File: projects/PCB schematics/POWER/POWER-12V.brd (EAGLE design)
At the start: 160 x 100 mm, 0 parts

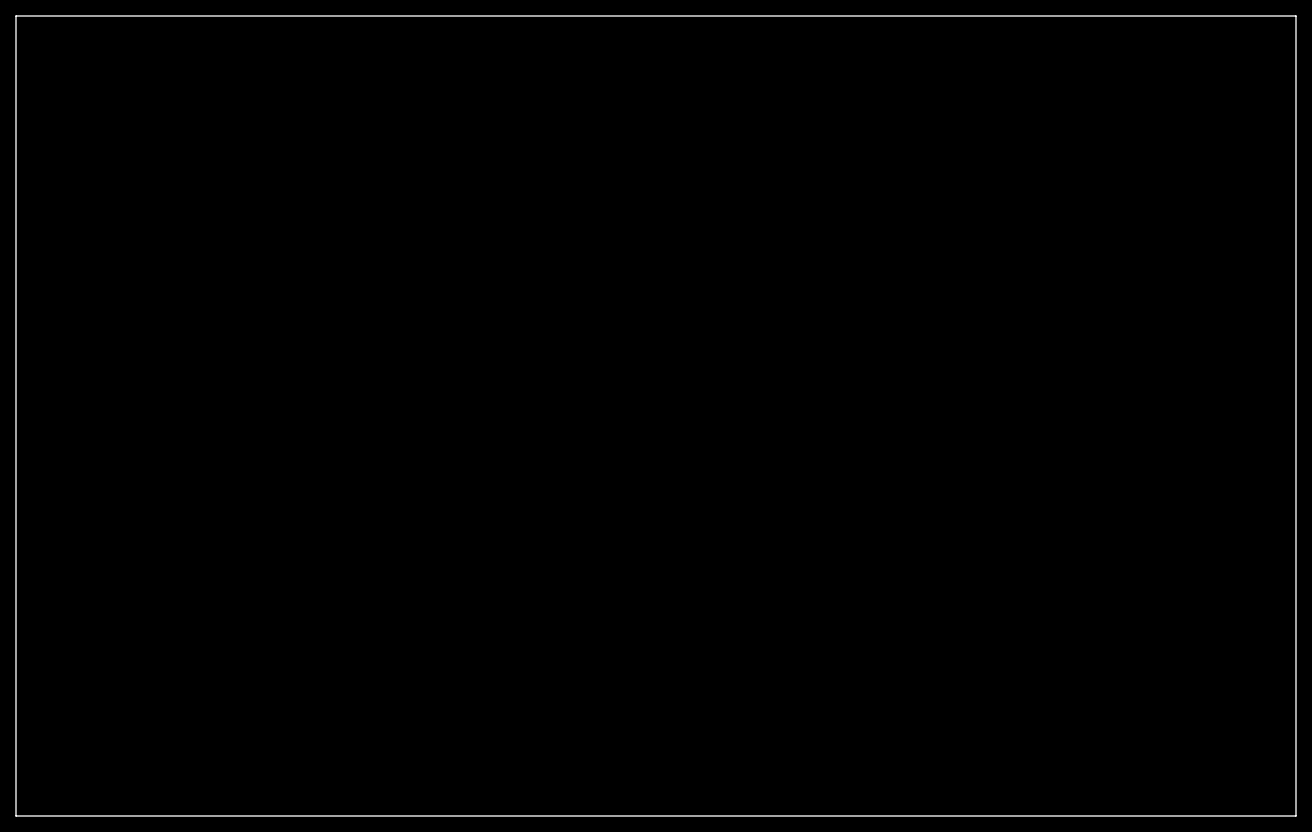
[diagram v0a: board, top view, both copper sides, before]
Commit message: RTDS - Rev A.
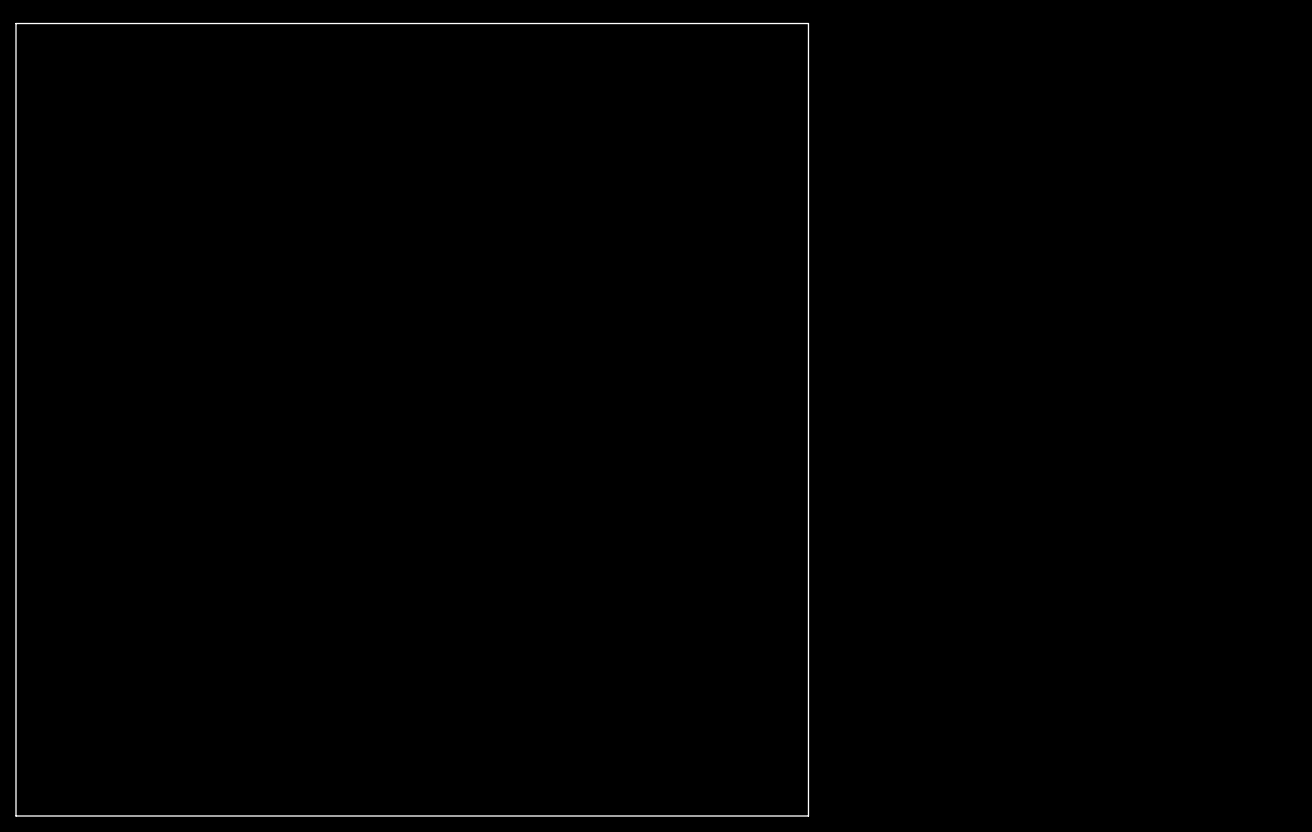
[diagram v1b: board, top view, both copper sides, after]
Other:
- board size 160 x 100 mm -> 99.1 x 99.1 mm
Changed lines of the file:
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@@
 <?xml version="1.0" encoding="utf-8"?>
 <!DOCTYPE eagle SYSTEM "eagle.dtd">
-<eagle version="9.3.2">
+<eagle version="9.4.0">
 <drawing>
 <settings>
@@
 <setting verticaltext="up"/>
 </settings>
-<grid distance="50" unitdist="mil" unit="mil" style="lines" multiple="1" display="no" altdistance="5" altunitdist="mil" altunit="mil"/>
+<grid distance="50" unitdist="mil" unit="mil" style="lines" multiple="1" display="yes" altdistance="1" altunitdist="mil" altunit="mil"/>
 <layers>
 <layer number="1" name="Top" color="4" fill="1" visible="yes" active="yes"/>
@@
 <board>
 <plain>
-<wire x1="0" y1="0" x2="160" y2="0" width="0" layer="20"/>
-<wire x1="160" y1="0" x2="160" y2="100" width="0" layer="20"/>
-<wire x1="160" y1="100" x2="0" y2="100" width="0" layer="20"/>
-<wire x1="0" y1="100" x2="0" y2="0" width="0" layer="20"/>
+<wire x1="0" y1="0" x2="99.06" y2="0" width="0" layer="20"/>
+<wire x1="99.06" y1="0" x2="99.06" y2="99.06" width="0" layer="20"/>
+<wire x1="99.06" y1="99.06" x2="0" y2="99.06" width="0" layer="20"/>
+<wire x1="0" y1="99.06" x2="0" y2="0" width="0" layer="20"/>
 </plain>
 <attributes>
@@
 </class>
 </classes>
-<designrules name="default">
-<description language="de">&lt;b&gt;EAGLE Design Rules&lt;/b&gt;
-&lt;p&gt;
-Die Standard-Design-Rules sind so gewählt, dass sie für
-die meisten Anwendungen passen. Sollte ihre Platine
-besondere Anforderungen haben, treffen Sie die erforderlichen
-Einstellungen hier und speichern die Design Rules unter
-einem neuen Namen ab.</description>
+<designrules name="default *">
 <description language="en">&lt;b&gt;EAGLE Design Rules&lt;/b&gt;
 &lt;p&gt;
@@
 <param name="mtCopper" value="0.035mm 0.035mm 0.035mm 0.035mm 0.035mm 0.035mm 0.035mm 0.035mm 0.035mm 0.035mm 0.035mm 0.035mm 0.035mm 0.035mm 0.035mm 0.035mm"/>
 <param name="mtIsolate" value="1.5mm 0.15mm 0.2mm 0.15mm 0.2mm 0.15mm 0.2mm 0.15mm 0.2mm 0.15mm 0.2mm 0.15mm 0.2mm 0.15mm 0.2mm"/>
-<param name="mdWireWire" value="6mil"/>
-<param name="mdWirePad" value="6mil"/>
-<param name="mdWireVia" value="6mil"/>
-<param name="mdPadPad" value="6mil"/>
-<param name="mdPadVia" value="6mil"/>
-<param name="mdViaVia" value="6mil"/>
-<param name="mdSmdPad" value="6mil"/>
-<param name="mdSmdVia" value="6mil"/>
-<param name="mdSmdSmd" value="6mil"/>
-<param name="mdViaViaSameLayer" value="6mil"/>
+<param name="mdWireWire" value="8mil"/>
+<param name="mdWirePad" value="8mil"/>
+<param name="mdWireVia" value="8mil"/>
+<param name="mdPadPad" value="8mil"/>
+<param name="mdPadVia" value="8mil"/>
+<param name="mdViaVia" value="8mil"/>
+<param name="mdSmdPad" value="8mil"/>
+<param name="mdSmdVia" value="8mil"/>
+<param name="mdSmdSmd" value="8mil"/>
+<param name="mdViaViaSameLayer" value="8mil"/>
 <param name="mnLayersViaInSmd" value="2"/>
-<param name="mdCopperDimension" value="40mil"/>
-<param name="mdDrill" value="6mil"/>
+<param name="mdCopperDimension" value="10mil"/>
+<param name="mdDrill" value="8mil"/>
 <param name="mdSmdStop" value="0mil"/>
-<param name="msWidth" value="6mil"/>
-<param name="msDrill" value="0.35mm"/>
+<param name="msWidth" value="8mil"/>
+<param name="msDrill" value="20mil"/>
 <param name="msMicroVia" value="9.99mm"/>
 <param name="msBlindViaRatio" value="0.5"/>
@@
 <param name="rvMicroViaOuter" value="0.25"/>
 <param name="rvMicroViaInner" value="0.25"/>
-<param name="rlMinPadTop" value="10mil"/>
+<param name="rlMinPadTop" value="12mil"/>
 <param name="rlMaxPadTop" value="20mil"/>
 <param name="rlMinPadInner" value="10mil"/>
 <param name="rlMaxPadInner" value="20mil"/>
-<param name="rlMinPadBottom" value="10mil"/>
+<param name="rlMinPadBottom" value="12mil"/>
 <param name="rlMaxPadBottom" value="20mil"/>
-<param name="rlMinViaOuter" value="8mil"/>
+<param name="rlMinViaOuter" value="10mil"/>
 <param name="rlMaxViaOuter" value="20mil"/>
-<param name="rlMinViaInner" value="8mil"/>
+<param name="rlMinViaInner" value="10mil"/>
 <param name="rlMaxViaInner" value="20mil"/>
 <param name="rlMinMicroViaOuter" value="4mil"/>
@@
 <param name="mlMinCreamFrame" value="0mil"/>
 <param name="mlMaxCreamFrame" value="0mil"/>
-<param name="mlViaStopLimit" value="0mil"/>
+<param name="mlViaStopLimit" value="25mil"/>
 <param name="srRoundness" value="0"/>
 <param name="srMinRoundness" value="0mil"/>
